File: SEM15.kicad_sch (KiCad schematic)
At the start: 57 parts, among them Q1 PMOS, Q2 Q_NMOS_DSG, Q5 AO3401A, Q6 PMOS, Q7 AO3401A, Q8 AO3401A, Q9 AO3401A, SW1 SW_DPST_x2, U1 STC8G1K08-SOP16

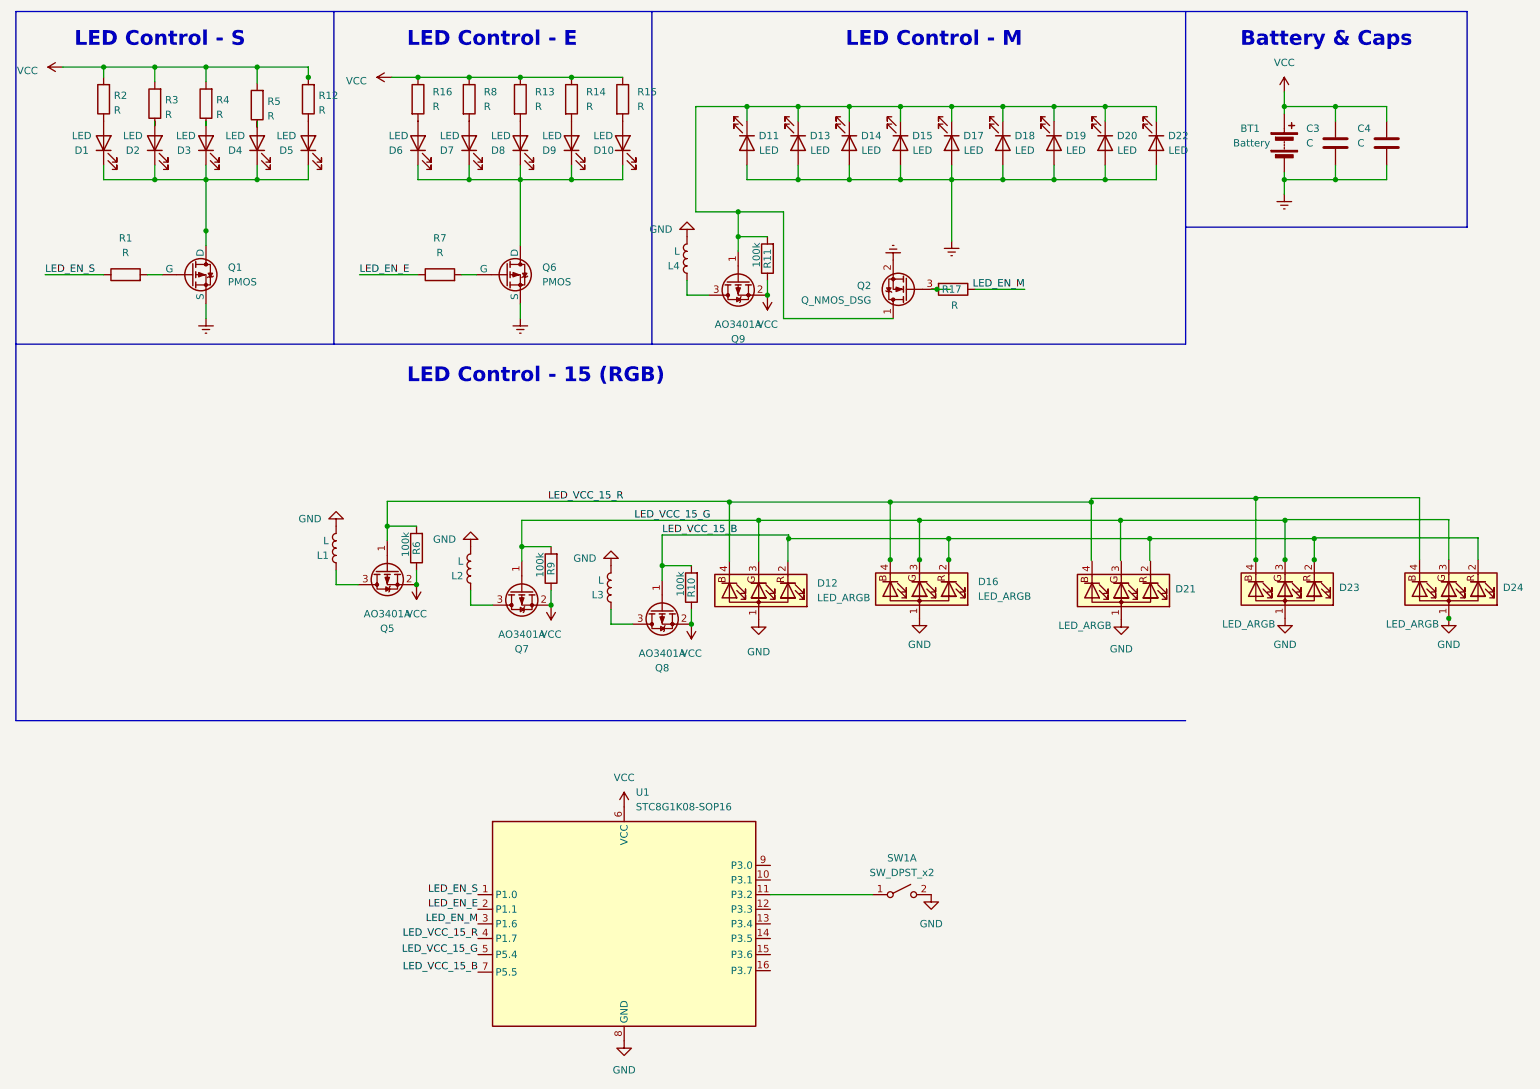
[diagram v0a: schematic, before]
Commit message: sch kesz
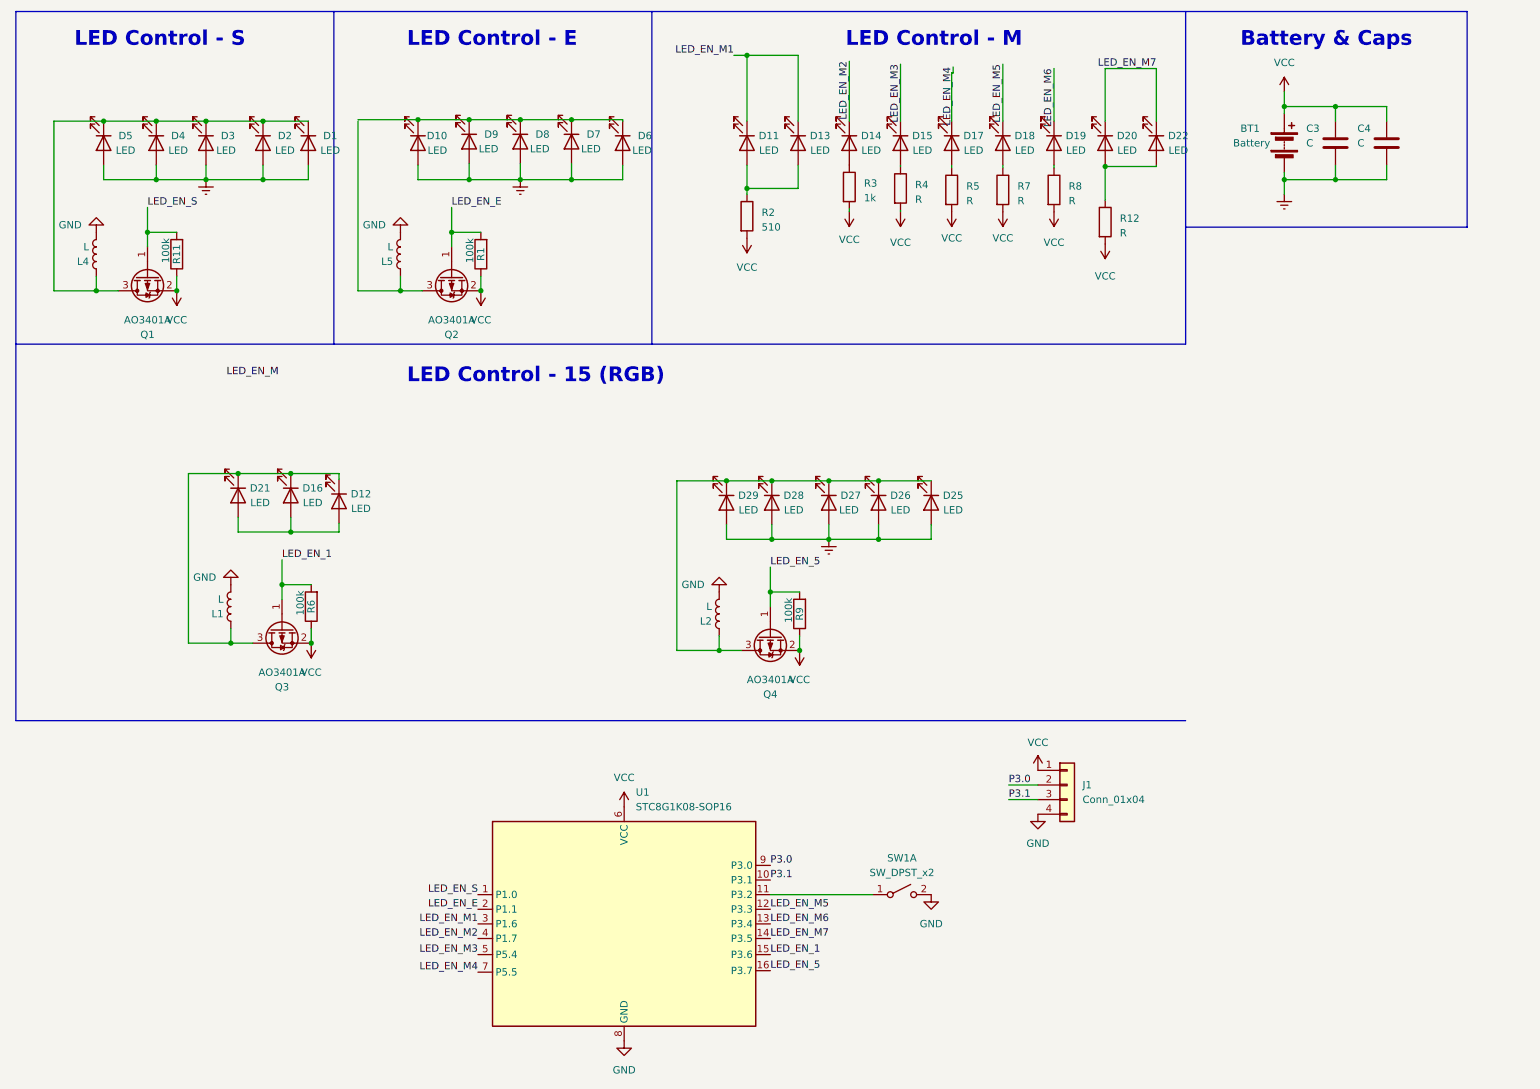
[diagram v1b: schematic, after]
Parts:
- removed D12, D16, D21, D23, D24: LED_ARGB, LED_SMD:LED_RGB_Wuerth-PLCC4_3.2x2.8mm_150141M173100, symbol Device:LED_ARGB
- removed L3: L, Inductor_SMD:L_1008_2520Metric, symbol Device:L
- removed Q1, Q6: PMOS, symbol Simulation_SPICE:PMOS
- removed Q2: Q_NMOS_DSG, symbol Device:Q_NMOS_DSG
- removed Q5, Q7, Q8, Q9: AO3401A, sajat:SOT-23, symbol Transistor_FET:AO3401A
- removed R10: 100k, Resistor_SMD:R_0603_1608Metric, symbol Device:R
- removed R13, R14, R15, R16, R17: R, Resistor_SMD:R_0603_1608Metric, symbol Device:R
- added D12, D16, D21, D25, D26, D27, D28, D29: LED, LED_SMD:LED_0805_2012Metric, symbol Device:LED
- added J1: Conn_01x04, Connector_PinHeader_1.27mm:PinHeader_1x04_P1.27mm_Vertical, symbol Connector_Generic:Conn_01x04
- added L5: L, Inductor_SMD:L_1008_2520Metric, symbol Device:L
- added Q1, Q2, Q3, Q4: AO3401A, sajat:SOT-23, symbol Transistor_FET:AO3401A
- R1: value R -> 100k
- R12, R4, R5, R7, R8: footprint Resistor_SMD:R_0603_1608Metric -> (none)
- R2: value R -> 510; footprint Resistor_SMD:R_0603_1608Metric -> (none)
- R3: value R -> 1k; footprint Resistor_SMD:R_0603_1608Metric -> (none)
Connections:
- net Earth: now also D1.2 (A), D10.2 (A), D2.2 (A), D3.2 (A), D4.2 (A), D5.2 (A), D6.2 (A), D7.2 (A), D8.2 (A), D9.2 (A), D25.2 (A), D26.2 (A), D27.2 (A), D28.2 (A), D29.2 (A); no longer D11.2 (A), D13.2 (A), D14.2 (A), D15.2 (A), D17.2 (A), D18.2 (A), D19.2 (A), D20.2 (A), D22.2 (A)
- net GND: now also J1.4 (Pin_4), L5.2
- net LED_EN_E: now also R1.2, Q2.1 (G); no longer R7.1
- net LED_EN_M: no longer U1.3 (P1.6)
- net LED_EN_S: now also R11.2, Q1.1 (G); no longer R1.1
- net VCC: now also R1.1, R7.2, R8.2, J1.1 (Pin_1), Q1.2 (S), Q2.2 (S), Q3.2 (S), Q4.2 (S); no longer R8.1
- net at L4.1: now also D1.1 (K), D2.1 (K), D3.1 (K), D4.1 (K), D5.1 (K), Q1.3 (D)
- net at L1.1: now also D12.1 (K), D16.1 (K), D21.1 (K), Q3.3 (D)
- net at R4.1: now also D15.2 (A); no longer D3.2 (A)
- net at R2.1: now also D11.2 (A), D13.2 (A); no longer D1.2 (A)
- net at R5.1: now also D17.2 (A); no longer D4.2 (A)
- net P3.1: now reaches U1.10 (P3.1)
- net P3.1: now also J1.3 (Pin_3)
- net LED_EN_M5: now reaches U1.12 (P3.3)
- net LED_EN_M5: now also D18.1 (K)
- net LED_EN_M6: now reaches U1.13 (P3.4)
- net LED_EN_M6: now also D19.1 (K)
- net LED_EN_M7: now reaches U1.14 (P3.5)
- net LED_EN_M7: now also D20.1 (K), D22.1 (K)
- net LED_EN_1: now reaches U1.15 (P3.6)
- net LED_EN_1: now also R6.2, Q3.1 (G)
- net LED_EN_5: now reaches U1.16 (P3.7)
- net LED_EN_5: now also R9.2, Q4.1 (G)
- net P3.0: now reaches U1.9 (P3.0)
- net P3.0: now also J1.2 (Pin_2)
- net at L2.1: now also D25.1 (K), D26.1 (K), D27.1 (K), D28.1 (K), D29.1 (K), Q4.3 (D)
- net at R3.1: now also D14.2 (A); no longer D2.2 (A)
- net at R12.1: now also D20.2 (A), D22.2 (A); no longer D5.2 (A)
- net LED_VCC_15_B renamed LED_EN_M4
- net LED_EN_M4: now also D17.1 (K)
- net LED_VCC_15_G renamed LED_EN_M3
- net LED_EN_M3: now also D15.1 (K); no longer R9.2
- net LED_VCC_15_R renamed LED_EN_M2
- net LED_EN_M2: now also D14.1 (K); no longer R6.2
- new net: L5.1, Q2.3 (D)
- new net: D18.2 (A), R7.1
- new net: D19.2 (A), R8.1
- new net: D12.2 (A), D16.2 (A), D21.2 (A)
- new net LED_EN_M1: D11.1 (K), D13.1 (K), U1.3 (P1.6)
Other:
- moved on the sheet: D1, D10, D2, D3, D4, D5, D6, D7, D8, D9
